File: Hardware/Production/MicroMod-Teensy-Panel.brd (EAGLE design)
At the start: 199.6 x 83.1 mm, 1142 parts, among them J1 MICROMOD-2222, J10 MICROMOD-2222, J11 MICROMOD-2222, J12 MICROMOD-2222, J13 MICROMOD-2222, J14 MICROMOD-2222, J15 MICROMOD-2222, J16 MICROMOD-2222, J2 MICROMOD-2222, J3 MICROMOD-2222, J4 MICROMOD-2222, J5 MICROMOD-2222, J6 MICROMOD-2222, J7 MICROMOD-2222, J8 MICROMOD-2222, J9 MICROMOD-2222, U1 IMXRT1062DV10X10, U10 IMXRT1062DV10X10, U11 W25QXX3X2, U12 MKL02Z32VFG4, U13 IMXRT1062DV10X10, U14 W25QXX3X2, U15 MKL02Z32VFG4, U16 IMXRT1062DV10X10, U17 W25QXX3X2, U18 MKL02Z32VFG4, U19 IMXRT1062DV10X10, U2 W25QXX3X2, U20 W25QXX3X2, U21 MKL02Z32VFG4, U22 IMXRT1062DV10X10, U23 W25QXX3X2, U24 MKL02Z32VFG4, U25 IMXRT1062DV10X10, U26 W25QXX3X2, U27 MKL02Z32VFG4, U28 IMXRT1062DV10X10, U29 W25QXX3X2, U3 MKL02Z32VFG4, U30 MKL02Z32VFG4, U31 IMXRT1062DV10X10, U32 W25QXX3X2, U33 MKL02Z32VFG4, U34 IMXRT1062DV10X10, U35 W25QXX3X2, U36 MKL02Z32VFG4, U37 IMXRT1062DV10X10, U38 W25QXX3X2, U39 MKL02Z32VFG4, U4 IMXRT1062DV10X10, U40 IMXRT1062DV10X10, U41 W25QXX3X2, U42 MKL02Z32VFG4, U43 IMXRT1062DV10X10, U44 W25QXX3X2, U45 MKL02Z32VFG4, U46 IMXRT1062DV10X10, U47 W25QXX3X2, U48 MKL02Z32VFG4, U5 W25QXX3X2, U6 MKL02Z32VFG4, U7 IMXRT1062DV10X10, U8 W25QXX3X2, U9 MKL02Z32VFG4, Y1 32.768kHz, Y10 24MHz, Y11 32.768kHz, Y12 24MHz, Y13 32.768kHz, Y14 24MHz, Y15 32.768kHz, Y16 24MHz, Y17 32.768kHz, Y18 24MHz, Y19 32.768kHz, Y2 24MHz, Y20 24MHz, Y21 32.768kHz, Y22 24MHz, Y23 32.768kHz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

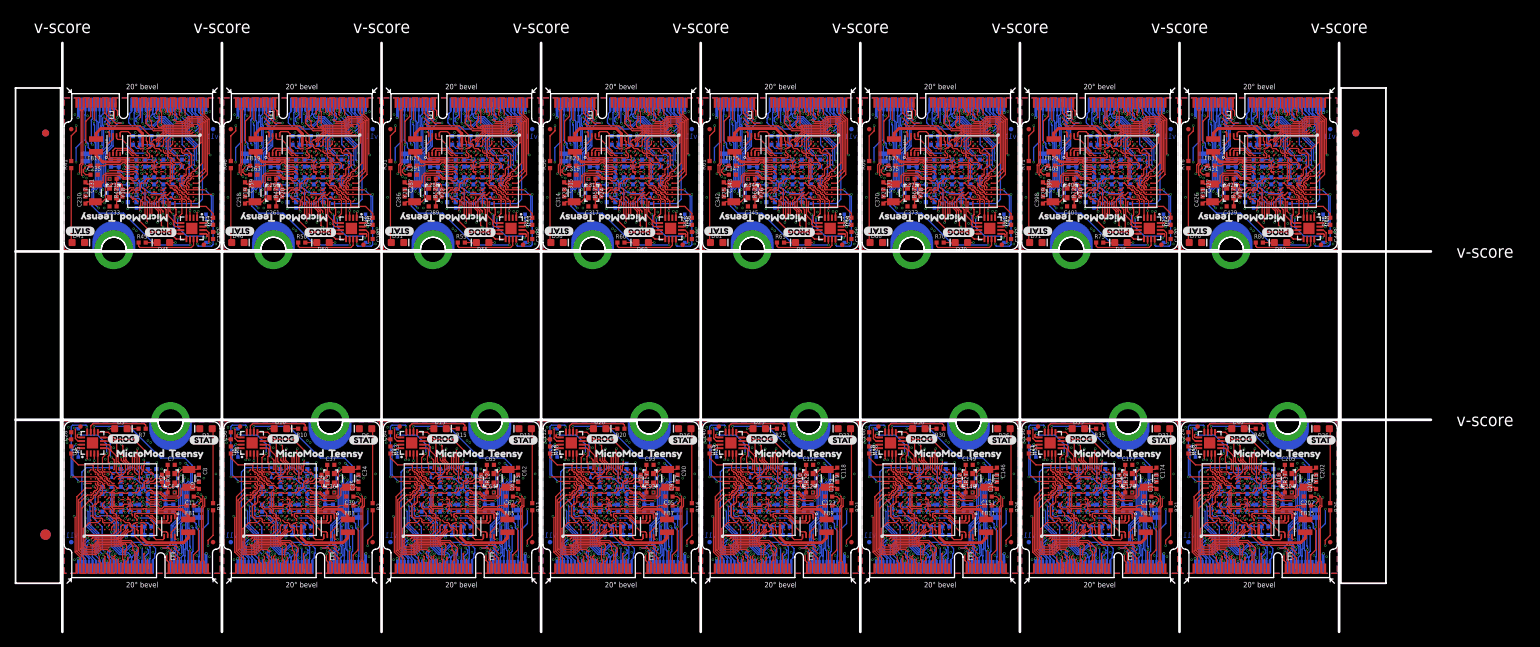
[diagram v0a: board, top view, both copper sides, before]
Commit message: Adding panel files
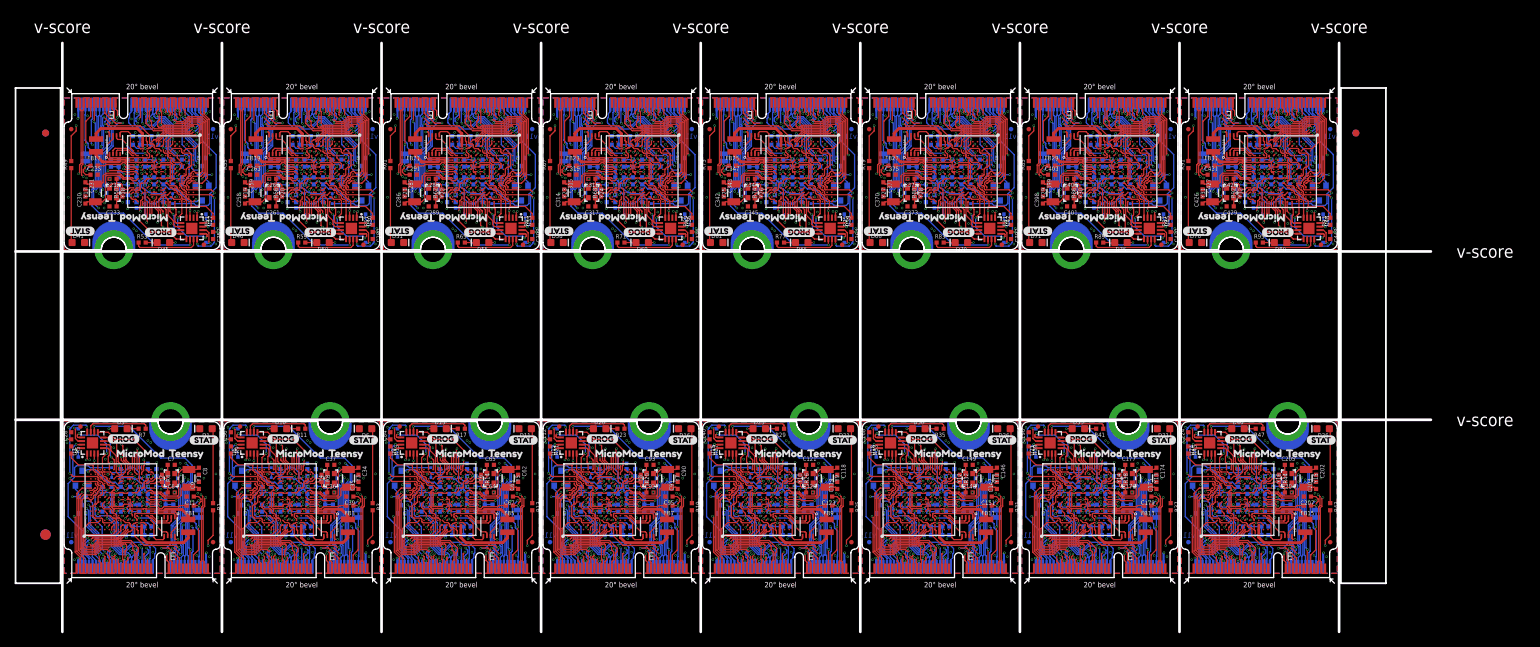
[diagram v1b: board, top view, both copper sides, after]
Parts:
- added Q1, Q11, Q13, Q15, Q17, Q19, Q21, Q23, Q25, Q27, Q29, Q3, Q31, Q5, Q7, Q9: 20V/4.2A/52mΩ/1.4W, SparkFun-DiscreteSemi:SOT23-3
- added Q10, Q12, Q14, Q16, Q18, Q2, Q20, Q22, Q24, Q26, Q28, Q30, Q32, Q4, Q6, Q8: 20V/0.2A/8MHz/1.2Ω/1Vth, SparkFun-DiscreteSemi:SOT-416FL
- added R81, R82, R84, R87, R88, R90, R93, R94, R96: 100k, SparkFun-Resistors:0402-TIGHT
- added R83, R85, R89, R91, R95: 1k, SparkFun-Resistors:0402-TIGHT
- added R86, R92: 2.2M, SparkFun-Resistors:0402-TIGHT
- R10, R15, R16, R2, R21, R30, R36, R40, R45, R46, R51, R60, R66, R70, R75, R76: value 1k -> 100k
- R12, R22, R27, R42, R52, R57, R72: value 2.2M -> 100k
- R13, R19, R23, R29, R43, R49, R53, R59, R73, R79: value 100k -> 1k
- R14, R38, R44, R68, R74, R8: value 100k -> 2.2M
- R17, R3, R37, R47, R67, R77: value 2.2M -> 1k
- R20, R26, R50, R56, R80: value 1k -> 2.2M
- moved R44 166.0 mm to (171.4, 14.8), flipped to the top
- moved R43 162.6 mm to (178.6, 10.8), turned to 270 degrees
- moved R46 152.5 mm to (168.2, 10.6), flipped to the bottom
- moved R45 150.4 mm to (158.6, 18.8), turned to 270 degrees
- moved R41 149.8 mm to (146.1, 21.8), turned to 180 degrees
- moved R47 141.8 mm to (168.6, 21.8), turned to 180 degrees
- moved R42 136.3 mm to (137.6, 12.2), flipped to the bottom, turned to 180 degrees
- moved R48 122.9 mm to (160.1, 12.2), flipped to the bottom, turned to 180 degrees
- moved R78 69.4 mm to (109.5, 57.6), flipped to the bottom, turned to 0 degrees
- moved R73 65.5 mm to (91.0, 59.0)
- moved R77 65.1 mm to (101.0, 48.0), turned to 0 degrees
- moved R36 63.5 mm to (115.1, 12.2), flipped to the bottom, turned to 180 degrees
- moved R71 58.6 mm to (78.5, 48.0), turned to 0 degrees
- moved R68 58.0 mm to (75.7, 55.0)
- moved R76 57.1 mm to (101.4, 59.2), flipped to the bottom, turned to 270 degrees
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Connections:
- removed net N$104 (its old number): C204.1, R37.2, U22.P11, Y16.1
- removed net N$11 (its old number): D6.A, R2.1
- removed net N$110 (its old number): R40.1, U24.11
- removed net N$116 (its old number): D41.A, R41.1
- removed net N$125 (its old number): D45.C, R45.2
- removed net N$130 (its old number): D46.A, R46.1
- removed net N$138 (its old number): R50.1, U30.11
- removed net N$144 (its old number): D51.A, R51.1
- removed net N$146 (its old number): C288.1, R52.2, U31.P11, Y22.1
- removed net N$15 (its old number): C36.1, R3.2, U4.P11, Y4.1
- removed net N$152 (its old number): R55.1, U33.11
- removed net N$153 (its old number): D55.C, R55.2
- removed net N$158 (its old number): D56.A, R56.1
- removed net N$160 (its old number): C316.1, R57.2, U34.P11, Y24.1
- removed net N$166 (its old number): R60.1, U36.11
- removed net N$167 (its old number): D60.C, R60.2
- removed net N$172 (its old number): D61.A, R61.1
- removed net N$174 (its old number): C344.1, R62.2, U37.P11, Y26.1
- removed net N$181 (its old number): D65.C, R65.2
- removed net N$188 (its old number): C372.1, R67.2, U40.P11, Y28.1
- removed net N$194 (its old number): R70.1, U42.11
- removed net N$200 (its old number): D71.A, R71.1
- removed net N$202 (its old number): C400.1, R72.2, U43.P11, Y30.1
- removed net N$209 (its old number): D75.C, R75.2
- removed net N$21 (its old number): R10.1, U6.11
- removed net N$27 (its old number): D11.A, R11.1
- removed net N$40 (its old number): R15.1, U9.11
- removed net N$41 (its old number): D15.C, R15.2
- removed net N$46 (its old number): D16.A, R16.1
- removed net N$48 (its old number): C92.1, R17.2, U10.P11, Y8.1
- removed net N$54 (its old number): R20.1, U12.11
- removed net N$55 (its old number): D20.C, R20.2
- removed net N$62 (its old number): C120.1, R22.2, U13.P11, Y10.1
- removed net N$68 (its old number): R25.1, U15.11
- removed net N$69 (its old number): D25.C, R25.2
- removed net N$74 (its old number): D26.A, R26.1
- removed net N$76 (its old number): C148.1, R27.2, U16.P11, Y12.1
- removed net N$82 (its old number): R30.1, U18.11
- removed net N$83 (its old number): D30.C, R30.2
- removed net N$97 (its old number): D35.C, R35.2
- new net 3.3V_CONTROLLED: C1.1, C2.1, C3.1, C4.1, C5.1, Q1.3, R6.1, U1.E6, U1.E9, U1.F10, U1.F5, U1.J10, U1.J6, U1.K4, U1.K5, U1.N14, U1.P12
- new net 3.3V_CONTROLLED1: C29.1, C30.1, C31.1, C32.1, C33.1, Q3.3, R10.1, U4.E6, U4.E9, U4.F10, U4.F5, U4.J10, U4.J6, U4.K4, U4.K5, U4.N14, U4.P12
- new net 3.3V_CONTROLLED10: C281.1, C282.1, C283.1, C284.1, C285.1, Q21.3, R64.1, U31.E6, U31.E9, U31.F10, U31.F5, U31.J10, U31.J6, U31.K4, U31.K5, U31.N14, U31.P12
- new net 3.3V_CONTROLLED11: C309.1, C310.1, C311.1, C312.1, C313.1, Q23.3, R70.1, U34.E6, U34.E9, U34.F10, U34.F5, U34.J10, U34.J6, U34.K4, U34.K5, U34.N14, U34.P12
- new net 3.3V_CONTROLLED12: C337.1, C338.1, C339.1, C340.1, C341.1, Q25.3, R76.1, U37.E6, U37.E9, U37.F10, U37.F5, U37.J10, U37.J6, U37.K4, U37.K5, U37.N14, U37.P12
- new net 3.3V_CONTROLLED13: C365.1, C366.1, C367.1, C368.1, C369.1, Q27.3, R82.1, U40.E6, U40.E9, U40.F10, U40.F5, U40.J10, U40.J6, U40.K4, U40.K5, U40.N14, U40.P12
- new net 3.3V_CONTROLLED14: C393.1, C394.1, C395.1, C396.1, C397.1, Q29.3, R88.1, U43.E6, U43.E9, U43.F10, U43.F5, U43.J10, U43.J6, U43.K4, U43.K5, U43.N14, U43.P12
- new net 3.3V_CONTROLLED15: C421.1, C422.1, C423.1, C424.1, C425.1, Q31.3, R94.1, U46.E6, U46.E9, U46.F10, U46.F5, U46.J10, U46.J6, U46.K4, U46.K5, U46.N14, U46.P12
- new net 3.3V_CONTROLLED2: C57.1, C58.1, C59.1, C60.1, C61.1, Q5.3, R16.1, U7.E6, U7.E9, U7.F10, U7.F5, U7.J10, U7.J6, U7.K4, U7.K5, U7.N14, U7.P12
- new net 3.3V_CONTROLLED3: C85.1, C86.1, C87.1, C88.1, C89.1, Q7.3, R22.1, U10.E6, U10.E9, U10.F10, U10.F5, U10.J10, U10.J6, U10.K4, U10.K5, U10.N14, U10.P12
- new net 3.3V_CONTROLLED4: C113.1, C114.1, C115.1, C116.1, C117.1, Q9.3, R28.1, U13.E6, U13.E9, U13.F10, U13.F5, U13.J10, U13.J6, U13.K4, U13.K5, U13.N14, U13.P12
- new net 3.3V_CONTROLLED5: C141.1, C142.1, C143.1, C144.1, C145.1, Q11.3, R34.1, U16.E6, U16.E9, U16.F10, U16.F5, U16.J10, U16.J6, U16.K4, U16.K5, U16.N14, U16.P12
- new net 3.3V_CONTROLLED6: C169.1, C170.1, C171.1, C172.1, C173.1, Q13.3, R40.1, U19.E6, U19.E9, U19.F10, U19.F5, U19.J10, U19.J6, U19.K4, U19.K5, U19.N14, U19.P12
- new net 3.3V_CONTROLLED7: C197.1, C198.1, C199.1, C200.1, C201.1, Q15.3, R46.1, U22.E6, U22.E9, U22.F10, U22.F5, U22.J10, U22.J6, U22.K4, U22.K5, U22.N14, U22.P12
- new net 3.3V_CONTROLLED8: C225.1, C226.1, C227.1, C228.1, C229.1, Q17.3, R52.1, U25.E6, U25.E9, U25.F10, U25.F5, U25.J10, U25.J6, U25.K4, U25.K5, U25.N14, U25.P12
- new net 3.3V_CONTROLLED9: C253.1, C254.1, C255.1, C256.1, C257.1, Q19.3, R58.1, U28.E6, U28.E9, U28.F10, U28.F5, U28.J10, U28.J6, U28.K4, U28.K5, U28.N14, U28.P12
- new net N$103: D35.C, R41.2
- new net N$105: Q13.1, Q14.3, R42.2
- new net N$109: D36.A, R43.1
- new net N$117: R47.1, U24.11
- new net N$120: Q15.1, Q16.3, R48.2
- new net N$126: C232.1, R50.2, U25.P11, Y18.1
- new net N$133: D45.C, R53.2
- new net N$135: Q17.1, Q18.3, R54.2
- new net N$14: D6.A, R3.1
- new net N$141: C260.1, R56.2, U28.P11, Y20.1
- new net N$147: R59.1, U30.11
- new net N$148: D50.C, R59.2
- new net N$150: Q19.1, Q20.3, R60.2
- new net N$154: D51.A, R61.1
- new net N$156: C288.1, R62.2, U31.P11, Y22.1
- new net N$16: C36.1, R8.2, U4.P11, Y4.1
- new net N$162: R65.1, U33.11
- new net N$163: D55.C, R65.2
- new net N$165: Q21.1, Q22.3, R66.2
- new net N$169: D56.A, R67.1
- new net N$171: C316.1, R68.2, U34.P11, Y24.1
- new net N$177: R71.1, U36.11
- new net N$178: D60.C, R71.2
- new net N$184: D61.A, R73.1
- new net N$192: R77.1, U39.11
- new net N$193: D65.C, R77.2
- new net N$199: D66.A, R79.1
- new net N$201: C372.1, R80.2, U40.P11, Y28.1
- new net N$207: R83.1, U42.11
- new net N$210: Q27.1, Q28.3, R84.2
- new net N$225: Q29.1, Q30.3, R90.2
- new net N$229: D76.A, R91.1
- new net N$23: D10.C, R11.2
- new net N$231: C428.1, R92.2, U46.P11, Y32.1
- new net N$237: R95.1, U48.11
- new net N$238: D80.C, R95.2
- new net N$240: Q31.1, Q32.3, R96.2
- new net N$25: Q3.1, Q4.3, R12.2
- new net N$36: C64.1, R14.2, U7.P11, Y6.1
- new net N$42: R17.1, U9.11
- new net N$43: D15.C, R17.2
- new net N$45: Q5.1, Q6.3, R18.2
- new net N$49: D16.A, R19.1
- new net N$51: C92.1, R20.2, U10.P11, Y8.1
- new net N$57: R23.1, U12.11
- new net N$58: D20.C, R23.2
- new net N$64: D21.A, R25.1
- new net N$66: C120.1, R26.2, U13.P11, Y10.1
- new net N$7: Q1.1, Q2.3, R2.2
- new net N$72: R29.1, U15.11
- new net N$73: D25.C, R29.2
- new net N$75: Q10.3, Q9.1, R30.2
- new net N$79: D26.A, R31.1
- new net N$81: C148.1, R32.2, U16.P11, Y12.1
- new net N$87: R35.1, U18.11
- new net N$94: D31.A, R37.1
- net 3.3V: now also Q1.2, R2.1; no longer C1.1, C2.1, C3.1, C4.1, C5.1, R6.1, U1.E6, U1.E9, U1.F10, U1.F5, U1.J10, U1.J6, U1.K4, U1.K5, U1.N14, U1.P12
- net 3.3V1: now also Q3.2, R12.1; no longer C29.1, C30.1, C31.1, C32.1, C33.1, R9.1, U4.E6, U4.E9, U4.F10, U4.F5, U4.J10, U4.J6, U4.K4, U4.K5, U4.N14, U4.P12
- net 3.3V10: now also Q21.2, R66.1; no longer C281.1, C282.1, C283.1, C284.1, C285.1, R54.1, U31.E6, U31.E9, U31.F10, U31.F5, U31.J10, U31.J6, U31.K4, U31.K5, U31.N14, U31.P12
- net 3.3V11: now also Q23.2, R72.1; no longer C309.1, C310.1, C311.1, C312.1, C313.1, R59.1, U34.E6, U34.E9, U34.F10, U34.F5, U34.J10, U34.J6, U34.K4, U34.K5, U34.N14, U34.P12
- net 3.3V12: now also Q25.2, R78.1; no longer C337.1, C338.1, C339.1, C340.1, C341.1, R64.1, U37.E6, U37.E9, U37.F10, U37.F5, U37.J10, U37.J6, U37.K4, U37.K5, U37.N14, U37.P12
- net 3.3V13: now also Q27.2, R84.1; no longer C365.1, C366.1, C367.1, C368.1, C369.1, R69.1, U40.E6, U40.E9, U40.F10, U40.F5, U40.J10, U40.J6, U40.K4, U40.K5, U40.N14, U40.P12
- net 3.3V14: now also Q29.2, R90.1; no longer C393.1, C394.1, C395.1, C396.1, C397.1, R74.1, U43.E6, U43.E9, U43.F10, U43.F5, U43.J10, U43.J6, U43.K4, U43.K5, U43.N14, U43.P12
- net 3.3V15: now also Q31.2, R96.1; no longer C421.1, C422.1, C423.1, C424.1, C425.1, R79.1, U46.E6, U46.E9, U46.F10, U46.F5, U46.J10, U46.J6, U46.K4, U46.K5, U46.N14, U46.P12
- net 3.3V2: now also Q5.2, R18.1; no longer C57.1, C58.1, C59.1, C60.1, C61.1, R14.1, U7.E6, U7.E9, U7.F10, U7.F5, U7.J10, U7.J6, U7.K4, U7.K5, U7.N14, U7.P12
- net 3.3V3: now also Q7.2, R24.1; no longer C85.1, C86.1, C87.1, C88.1, C89.1, R19.1, U10.E6, U10.E9, U10.F10, U10.F5, U10.J10, U10.J6, U10.K4, U10.K5, U10.N14, U10.P12
- net 3.3V4: now also Q9.2, R30.1; no longer C113.1, C114.1, C115.1, C116.1, C117.1, R24.1, U13.E6, U13.E9, U13.F10, U13.F5, U13.J10, U13.J6, U13.K4, U13.K5, U13.N14, U13.P12
- net 3.3V5: now also Q11.2, R36.1; no longer C141.1, C142.1, C143.1, C144.1, C145.1, R29.1, U16.E6, U16.E9, U16.F10, U16.F5, U16.J10, U16.J6, U16.K4, U16.K5, U16.N14, U16.P12
- net 3.3V6: now also Q13.2, R42.1; no longer C169.1, C170.1, C171.1, C172.1, C173.1, R34.1, U19.E6, U19.E9, U19.F10, U19.F5, U19.J10, U19.J6, U19.K4, U19.K5, U19.N14, U19.P12
- net 3.3V7: now also Q15.2, R48.1; no longer C197.1, C198.1, C199.1, C200.1, C201.1, R39.1, U22.E6, U22.E9, U22.F10, U22.F5, U22.J10, U22.J6, U22.K4, U22.K5, U22.N14, U22.P12
- net 3.3V8: now also Q17.2, R54.1; no longer C225.1, C226.1, C227.1, C228.1, C229.1, R44.1, U25.E6, U25.E9, U25.F10, U25.F5, U25.J10, U25.J6, U25.K4, U25.K5, U25.N14, U25.P12
- net 3.3V9: now also Q19.2, R60.1; no longer C253.1, C254.1, C255.1, C256.1, C257.1, R49.1, U28.E6, U28.E9, U28.F10, U28.F5, U28.J10, U28.J6, U28.K4, U28.K5, U28.N14, U28.P12
- net GND: now also Q2.2
- net GND1: now also Q4.2, R9.1; no longer R3.1
- net GND10: now also Q22.2, R62.1, R63.1; no longer R52.1, R53.1
- net GND11: now also Q24.2, R68.1, R69.1; no longer R57.1, R58.1
- net GND12: now also Q26.2, R74.1, R75.1; no longer R62.1, R63.1
- net GND13: now also Q28.2, R80.1, R81.1; no longer R67.1, R68.1
- net GND14: now also Q30.2, R86.1, R87.1; no longer R72.1, R73.1
- net GND15: now also Q32.2, R92.1, R93.1; no longer R77.1, R78.1
- net GND2: now also Q6.2, R14.1, R15.1; no longer R12.1, R13.1
- net GND3: now also Q8.2, R20.1, R21.1; no longer R17.1, R18.1
- net GND4: now also Q10.2, R26.1, R27.1; no longer R22.1, R23.1
- net GND5: now also Q12.2, R32.1, R33.1; no longer R27.1, R28.1
- net GND6: now also Q14.2, R38.1, R39.1; no longer R32.1, R33.1
- net GND7: now also Q16.2, R44.1, R45.1; no longer R37.1, R38.1
- net GND8: now also Q18.2, R50.1, R51.1; no longer R42.1, R43.1
- net GND9: now also Q20.2, R56.1, R57.1; no longer R47.1, R48.1
- net JTAG_TRST1: now also R9.2; no longer R8.2
- net JTAG_TRST10: now also R63.2; no longer R53.2
- net JTAG_TRST11: now also R69.2; no longer R58.2
- net JTAG_TRST12: now also R75.2; no longer R63.2
- net JTAG_TRST13: now also R81.2; no longer R68.2
- net JTAG_TRST14: now also R87.2; no longer R73.2
- net JTAG_TRST15: now also R93.2; no longer R78.2
- net JTAG_TRST2: now also R15.2; no longer R13.2
- net JTAG_TRST3: now also R21.2; no longer R18.2
- net JTAG_TRST4: now also R27.2; no longer R23.2
- net JTAG_TRST5: now also R33.2; no longer R28.2
- net JTAG_TRST6: now also R39.2; no longer R33.2
- net JTAG_TRST7: now also R45.2; no longer R38.2
- net JTAG_TRST8: now also R51.2; no longer R43.2
- net JTAG_TRST9: now also R57.2; no longer R48.2
- net N$102: now also R41.1, U21.11; no longer D36.A, R36.1
- net N$111: now also C204.1, R44.2, U22.P11, Y16.1; no longer D40.C, R40.2
- net N$118: now also D40.C, R47.2; no longer C232.1, R42.2, U25.P11, Y18.1
- net N$124: now also D41.A, R49.1; no longer R45.1, U27.11
- net N$132: now also R53.1, U27.11; no longer C260.1, R47.2, U28.P11, Y20.1
- net N$139: now also D46.A, R55.1; no longer D50.C, R50.2
- net N$180: now also Q23.1, Q24.3, R72.2; no longer R65.1, U39.11
- net N$186: now also C344.1, R74.2, U37.P11, Y26.1; no longer D66.A, R66.1
- net N$195: now also Q25.1, Q26.3, R78.2; no longer D70.C, R70.2
- net N$208: now also D70.C, R83.2; no longer R75.1, U45.11
- net N$214: now also D71.A, R85.1; no longer D76.A, R76.1
- net N$216: now also C400.1, R86.2, U43.P11, Y30.1; no longer C428.1, R77.2, U46.P11, Y32.1
- net N$22: now also R11.1, U6.11; no longer D10.C, R10.2
- net N$222: now also R89.1, U45.11; no longer R80.1, U48.11
- net N$223: now also D75.C, R89.2; no longer D80.C, R80.2
- net N$29: now also D11.A, R13.1; no longer C64.1, R12.2, U7.P11, Y6.1
- net N$60: now also Q7.1, Q8.3, R24.2; no longer D21.A, R21.1
- net N$88: now also D30.C, R35.2; no longer D31.A, R31.1
- net N$90: now also Q11.1, Q12.3, R36.2; no longer C176.1, R32.2, U19.P11, Y14.1
- net N$96: now also C176.1, R38.2, U19.P11, Y14.1; no longer R35.1, U21.11
- net PMIC: now also Q2.1; no longer J1.4
- net PMIC1: now also Q4.1, R10.2; no longer J2.4, R9.2
- net PMIC10: now also Q22.1, R64.2; no longer J11.4, R54.2
- net PMIC11: now also Q24.1, R70.2; no longer J12.4, R59.2
- net PMIC12: now also Q26.1, R76.2; no longer J13.4, R64.2
- net PMIC13: now also Q28.1, R82.2; no longer J14.4, R69.2
- net PMIC14: now also Q30.1, R88.2; no longer J15.4, R74.2
- net PMIC15: now also Q32.1, R94.2; no longer J16.4, R79.2
- net PMIC2: now also Q6.1, R16.2; no longer J3.4, R14.2
- net PMIC3: now also Q8.1, R22.2; no longer J4.4, R19.2
- net PMIC4: now also Q10.1, R28.2; no longer J5.4, R24.2
- net PMIC5: now also Q12.1, R34.2; no longer J6.4, R29.2
- net PMIC6: now also Q14.1, R40.2; no longer J7.4, R34.2
- net PMIC7: now also Q16.1, R46.2; no longer J8.4, R39.2
- net PMIC8: now also Q18.1, R52.2; no longer J9.4, R44.2
- net PMIC9: now also Q20.1, R58.2; no longer J10.4, R49.2
- net SCK/1: now also R3.2; no longer R2.2
- net SCK/10: now also R61.2; no longer R51.2
- net SCK/11: now also R67.2; no longer R56.2
- net SCK/12: now also R73.2; no longer R61.2
- net SCK/14: now also R79.2; no longer R66.2
- net SCK/15: now also R85.2; no longer R71.2
- net SCK/16: now also R91.2; no longer R76.2
- net SCK/2: now also R13.2; no longer R11.2
- net SCK/3: now also R19.2; no longer R16.2
- net SCK/4: now also R25.2; no longer R21.2
- net SCK/5: now also R31.2; no longer R26.2
- net SCK/6: now also R37.2; no longer R31.2
- net SCK/7: now also R43.2; no longer R36.2
- net SCK/8: now also R49.2; no longer R41.2
- net SCK/9: now also R55.2; no longer R46.2
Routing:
- net 3.3V_CONTROLLED1: track 0.00 -> 28.6 mm, vias 0 -> 5
- net 3.3V_CONTROLLED6: track 0.00 -> 28.6 mm, vias 0 -> 5
- net 3.3V_CONTROLLED3: track 0.00 -> 28.6 mm, vias 0 -> 5
- net 3.3V_CONTROLLED7: track 0.00 -> 28.6 mm, vias 0 -> 5
- net 3.3V_CONTROLLED15: track 0.00 -> 28.6 mm, vias 0 -> 5
- net 3.3V_CONTROLLED10: track 0.00 -> 28.6 mm, vias 0 -> 5
- net 3.3V_CONTROLLED: track 0.00 -> 28.6 mm, vias 0 -> 5
- net 3.3V_CONTROLLED5: track 0.00 -> 28.6 mm, vias 0 -> 5
- net 3.3V_CONTROLLED14: track 0.00 -> 28.6 mm, vias 0 -> 5
- net 3.3V_CONTROLLED8: track 0.00 -> 28.6 mm, vias 0 -> 5
- net 3.3V_CONTROLLED4: track 0.00 -> 28.6 mm, vias 0 -> 5
- net 3.3V_CONTROLLED9: track 0.00 -> 28.6 mm, vias 0 -> 5
- net 3.3V_CONTROLLED2: track 0.00 -> 28.6 mm, vias 0 -> 5
- net 3.3V_CONTROLLED12: track 0.00 -> 28.6 mm, vias 0 -> 5
- net 3.3V_CONTROLLED11: track 0.00 -> 28.6 mm, vias 0 -> 5
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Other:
- outline, holes or cut-outs redrawn
